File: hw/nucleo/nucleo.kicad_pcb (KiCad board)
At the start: 2 copper layers, 71.1 x 55.9 mm, 26 parts, among them J1 Rain, J2 Wind, J3 GPS, J4 BMP280, J5 Power, J6 Light, J7 I2C1, J8 I2C2, U1 MIC550X, U2 NUCLEO_L476RG, U3 XBEE_S2C

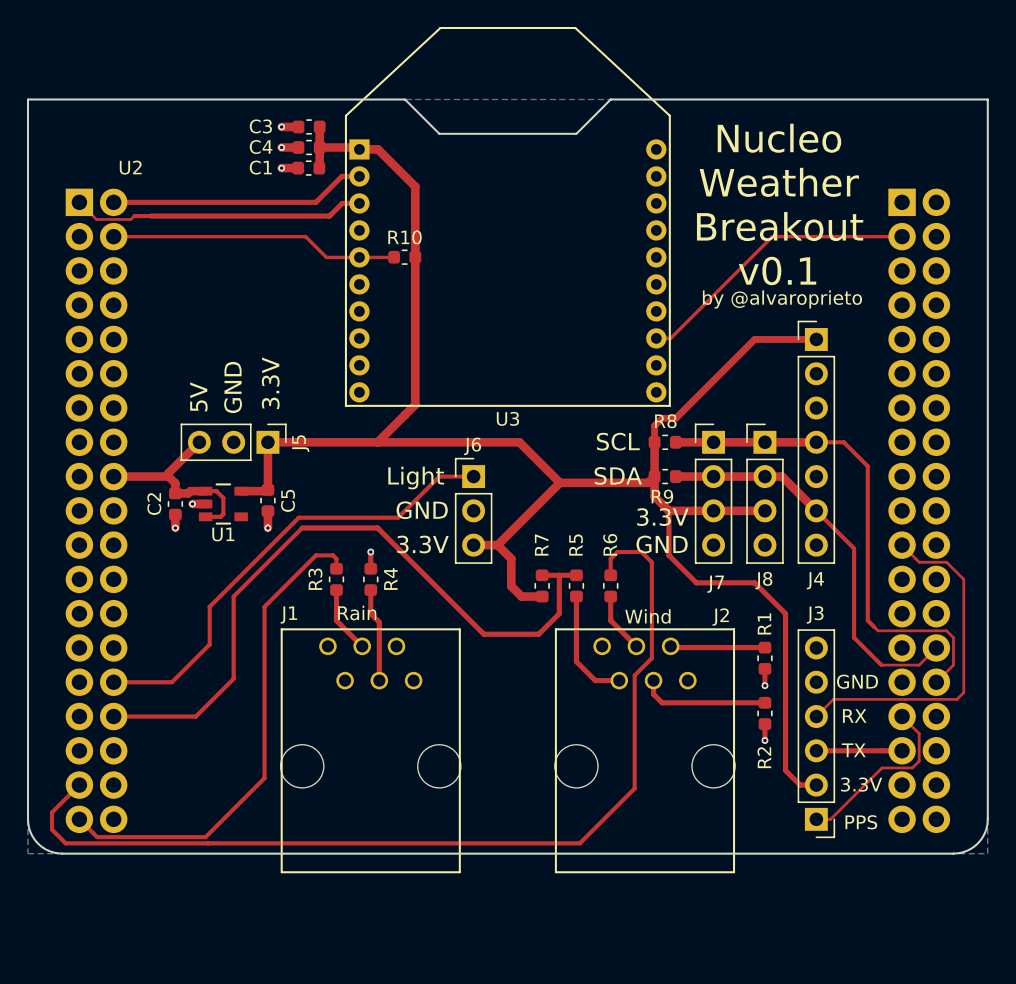
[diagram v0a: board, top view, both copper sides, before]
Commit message: Layout pretty much done. Time to review!
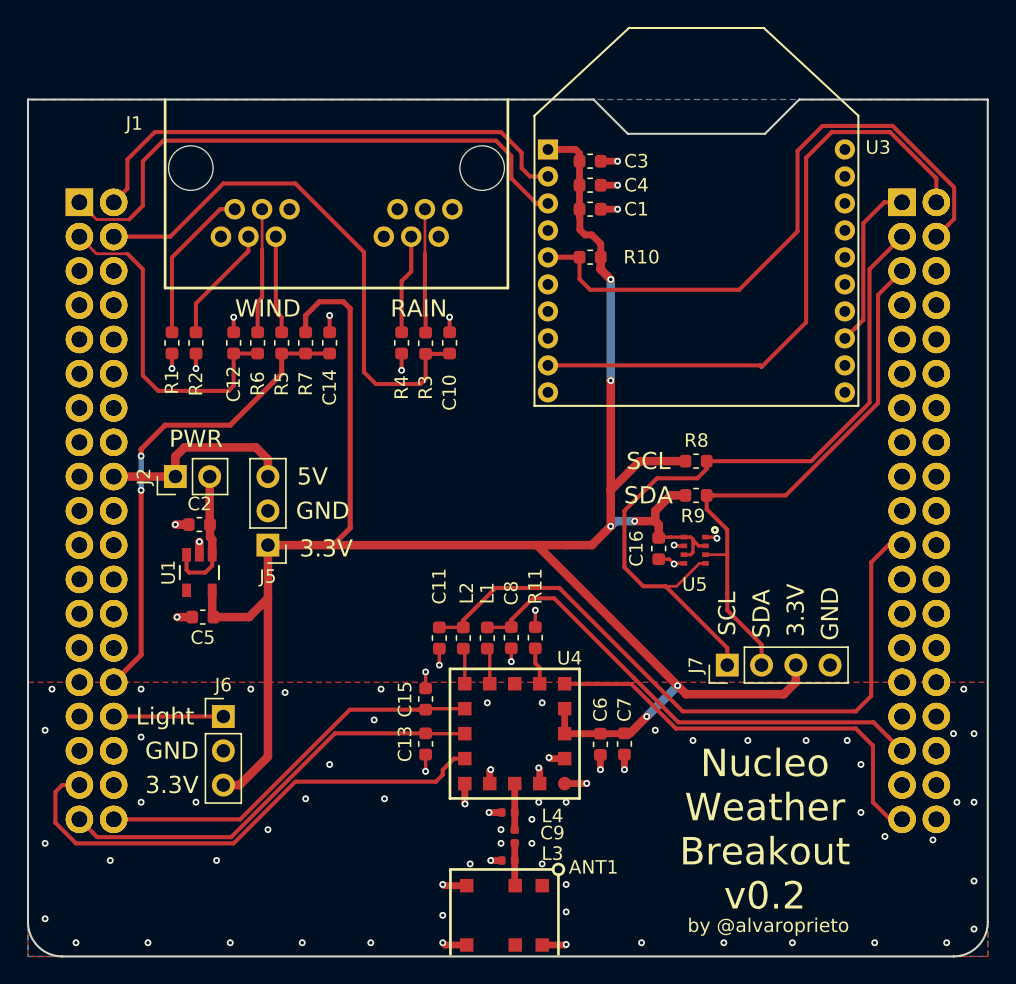
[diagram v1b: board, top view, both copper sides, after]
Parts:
- removed J3: GPS, Connector_PinHeader_2.54mm:PinHeader_1x06_P2.54mm_Vertical
- removed J4: BMP280, Connector_PinHeader_2.54mm:PinHeader_1x07_P2.54mm_Vertical
- removed J8: I2C2, Connector_PinHeader_2.54mm:PinHeader_1x04_P2.54mm_Vertical
- added ANT1: SR4G008, alvarop:SR4G008, F.Cu at (147.1, 139.2)
- added C10: 1nF, Capacitor_SMD:C_0603_1608Metric, F.Cu at (143.0, 96.8)
- added C11: 22pF, Capacitor_SMD:C_0603_1608Metric, F.Cu at (142.2, 118.6)
- added C12: 1nF, Capacitor_SMD:C_0603_1608Metric, F.Cu at (127.0, 96.8)
- added C13: 22pF, Capacitor_SMD:C_0603_1608Metric, F.Cu at (141.2, 126.5)
- added C14: 1nF, Capacitor_SMD:C_0603_1608Metric, F.Cu at (134.1, 96.8)
- added C15: 22pF, Capacitor_SMD:C_0603_1608Metric, F.Cu at (141.2, 123.2)
- added C16: 0.1uF, Capacitor_SMD:C_0603_1608Metric, F.Cu at (158.5, 112.0)
- added C6: 22pF, Capacitor_SMD:C_0603_1608Metric, F.Cu at (154.2, 126.5)
- added C7: 2.2uF, Capacitor_SMD:C_0603_1608Metric, F.Cu at (156.0, 126.5)
- added C8: 22pF, Capacitor_SMD:C_0603_1608Metric, F.Cu at (147.6, 118.6)
- added C9: 22pF, Capacitor_SMD:C_0402_1005Metric, F.Cu at (147.8, 133.3)
- added L1: 47nH, Inductor_SMD:L_0603_1608Metric, F.Cu at (145.8, 118.6)
- added L2: 47nH, Inductor_SMD:L_0603_1608Metric, F.Cu at (144.0, 118.6)
- added L3: DNP, Inductor_SMD:L_0402_1005Metric, F.Cu at (147.3, 135.1)
- added L4: DNP, Inductor_SMD:L_0402_1005Metric, F.Cu at (147.3, 131.6)
- added R11: 10k, Resistor_SMD:R_0603_1608Metric, F.Cu at (149.4, 118.6)
- added U2: NUCLEO_L476RG, alvarop:NUCLEO_L476RG, F.Cu at (147.3, 109.2)
- added U4: M10578-A2, alvarop:M10578-A2, F.Cu at (147.8, 125.7)
- added U5: BMP280, alvarop:BMP280, F.Cu at (161.2, 112.1)
- J1: value Rain -> windrain; footprint alvarop:RJ11 -> alvarop:043814-6621
- J2: value Wind -> Conn_01x02; footprint alvarop:RJ11 -> Connector_PinHeader_2.54mm:PinHeader_1x02_P2.54mm_Vertical
- J7: value I2C1 -> AM2315
- moved R2 50.3 mm to (124.2, 96.8)
- moved R1 49.8 mm to (122.4, 96.8), turned to 270 degrees
- moved J1 43.3 mm to (134.6, 83.8), turned to 180 degrees
- moved J2 40.3 mm to (122.7, 106.7), turned to 90 degrees
- moved R6 31.8 mm to (128.8, 96.8), turned to 90 degrees
- moved R5 28.3 mm to (130.6, 96.8), turned to 90 degrees
- moved J6 25.7 mm to (126.2, 124.5)
- moved R7 25.1 mm to (132.3, 96.8), turned to 90 degrees
- moved C1 21.1 mm to (153.4, 86.9), turned to 0 degrees
- moved C4 21.0 mm to (153.4, 85.1), turned to 0 degrees
- moved C3 21.0 mm to (153.4, 83.3), turned to 0 degrees
- moved R3 18.7 mm to (141.2, 96.8), turned to 90 degrees
- moved R4 17.7 mm to (139.4, 96.8)
- moved J7 16.5 mm to (163.6, 120.7), turned to 90 degrees
- moved U3 14.0 mm to (161.3, 91.4)
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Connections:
- C2 pad 1: /5V -> Net-(C2-Pad1)
- J2 pad 1: Net-(J2-Pad1) -> /5V
- J2 pad 2: Net-(J2-Pad2) -> Net-(C2-Pad1)
- R1 pad 1: GND -> Net-(J1-Pad11)
- R1 pad 2: Net-(J2-Pad5) -> GND
- R2 pad 2: Net-(J2-Pad4) -> Net-(J1-Pad10)
- R4 pad 1: GND -> Net-(J1-Pad4)
- R4 pad 2: Net-(J1-Pad4) -> GND
- R5 pad 2: Net-(J2-Pad2) -> Net-(J1-Pad8)
- R6 pad 2: Net-(J2-Pad3) -> Net-(J1-Pad9)
- U1 pad 1: /5V -> Net-(C2-Pad1)
- U1 pad 3: /5V -> Net-(C2-Pad1)
- U2 pad 3: Net-(U2-Pad3) -> /WSPEED
- U2 pad 30: /LIGHT -> /WDIR
- U2 pad 32: /WDIR -> /LIGHT
- U2 pad 35: /WSPEED -> /GPS_PPS
- U2 pad 37: /RAIN -> /GPS_nRST
- U2 pad 38: Net-(U2-Pad38) -> /GPS_SBY
- U2 pad 39: Net-(U2-Pad39) -> /XB_ON
- U2 pad 4: /XB_nRST -> /RAIN
- U2 pad 40: Net-(U2-Pad40) -> /XB_nSBY
- U2 pad 41: /XB_ON -> /SCL
- U2 pad 42: Net-(U2-Pad42) -> /XB_nRST
- U2 pad 43: Net-(U2-Pad43) -> /SDA
- U2 pad 66: /SDA -> Net-(U2-Pad66)
- U2 pad 68: /SCL -> Net-(U2-Pad68)
- U2 pad 69: /GPS_PPS -> Net-(U2-Pad69)
- U2 pad 75: Net-(U2-Pad75) -> /GPS_FIX
- U3 pad 9: Net-(U3-Pad9) -> /XB_nSBY
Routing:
- net /WSPEED: track 71.5 -> 25.1 mm
- net /XB_nSBY: track 0.00 -> 46.4 mm
- net /GPS_nRST: track 0.00 -> 32.3 mm
- net /GPS_FIX: track 0.00 -> 31.6 mm
- net /GPS_TXD: track 6.35 -> 36.6 mm
- net /GPS_SBY: track 0.00 -> 29.4 mm
- net GND: track 10.6 -> 39.1 mm, vias 9 -> 89
- net /LIGHT: track 34.6 -> 8.13 mm
- net +3V3: track 138.0 -> 164.3 mm, vias 0 -> 6
- net /XB_nRST: track 21.4 -> 46.7 mm
- net /GPS_RXD: track 25.7 -> 50.5 mm
- net /GPS_PPS: track 13.2 -> 38.1 mm
- net /XB_RX: track 21.8 -> 42.7 mm
- net /XB_TX: track 19.0 -> 37.6 mm
- net /SCL: track 37.1 -> 54.3 mm
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- added copper zone on F.Cu, net GND
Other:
- board size 71.1 x 55.9 mm -> 71.1 x 63.5 mm
- board text added: "Nucleo Weather Breakout v0.2"
- board text added: "PWR"
- board text added: "RAIN"
- board text added: "WIND"
- board text removed: "Nucleo Weather Breakout v0.1"
- board text removed: "PPS"
- board text removed: "RX"
- board text removed: "Rain"
- board text removed: "TX"
- board text removed: "Wind"
